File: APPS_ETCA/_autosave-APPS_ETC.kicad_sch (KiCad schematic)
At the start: 7 parts, among them U1 NUCLEO-L432KC, U2 ISO1050DUB, U3 A1365xKTTN-1, U4 A1365xKTTN-1, U5 L78S05CV

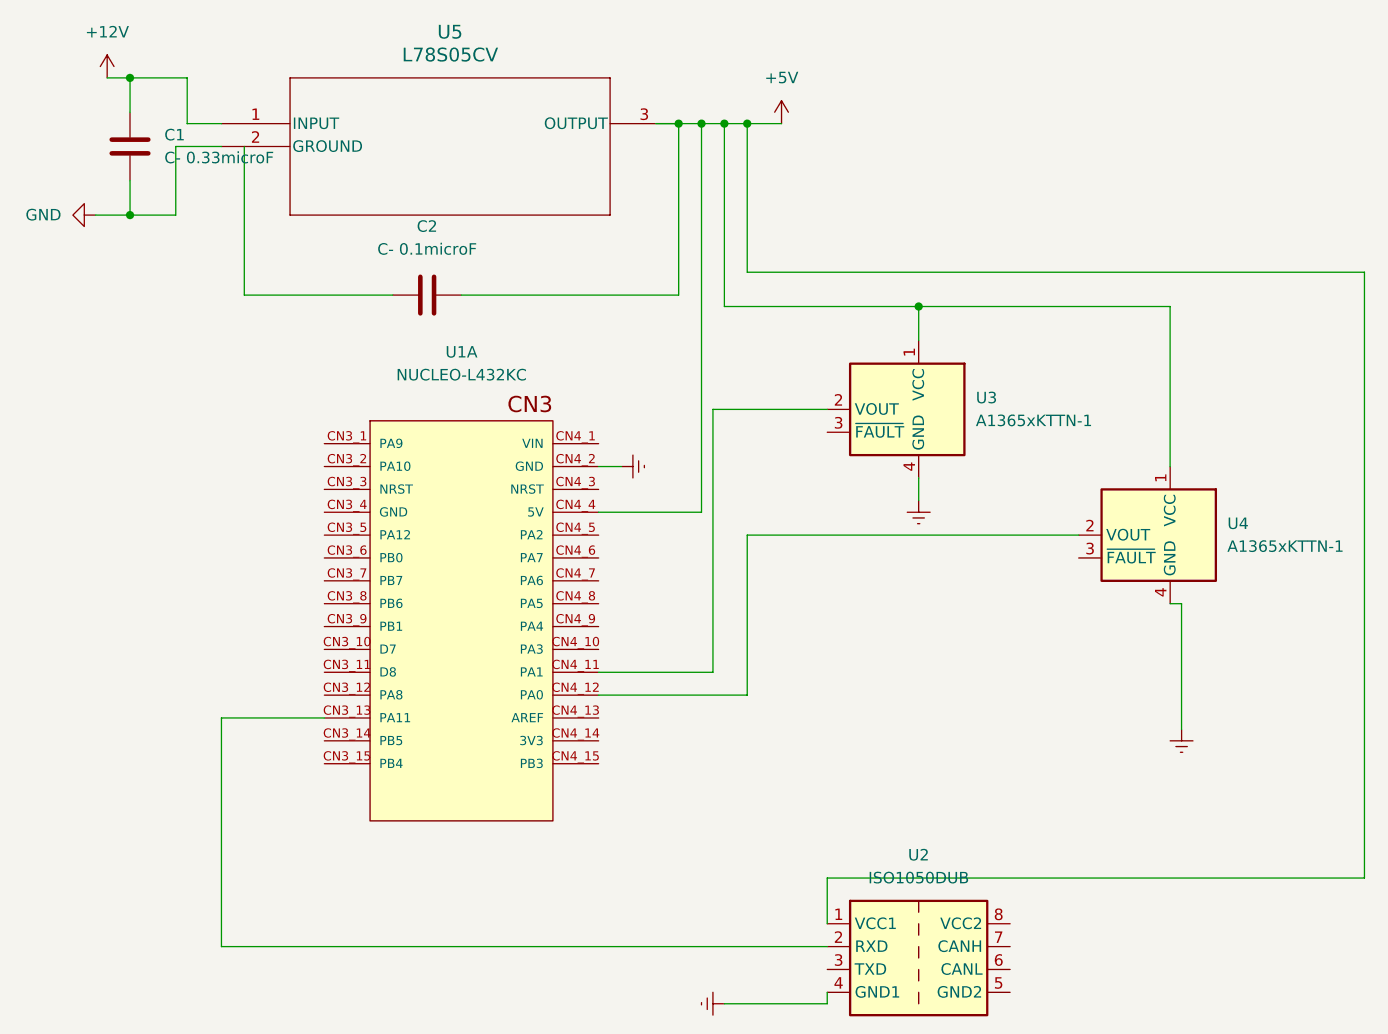
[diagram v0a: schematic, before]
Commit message: schema updates - making progress!
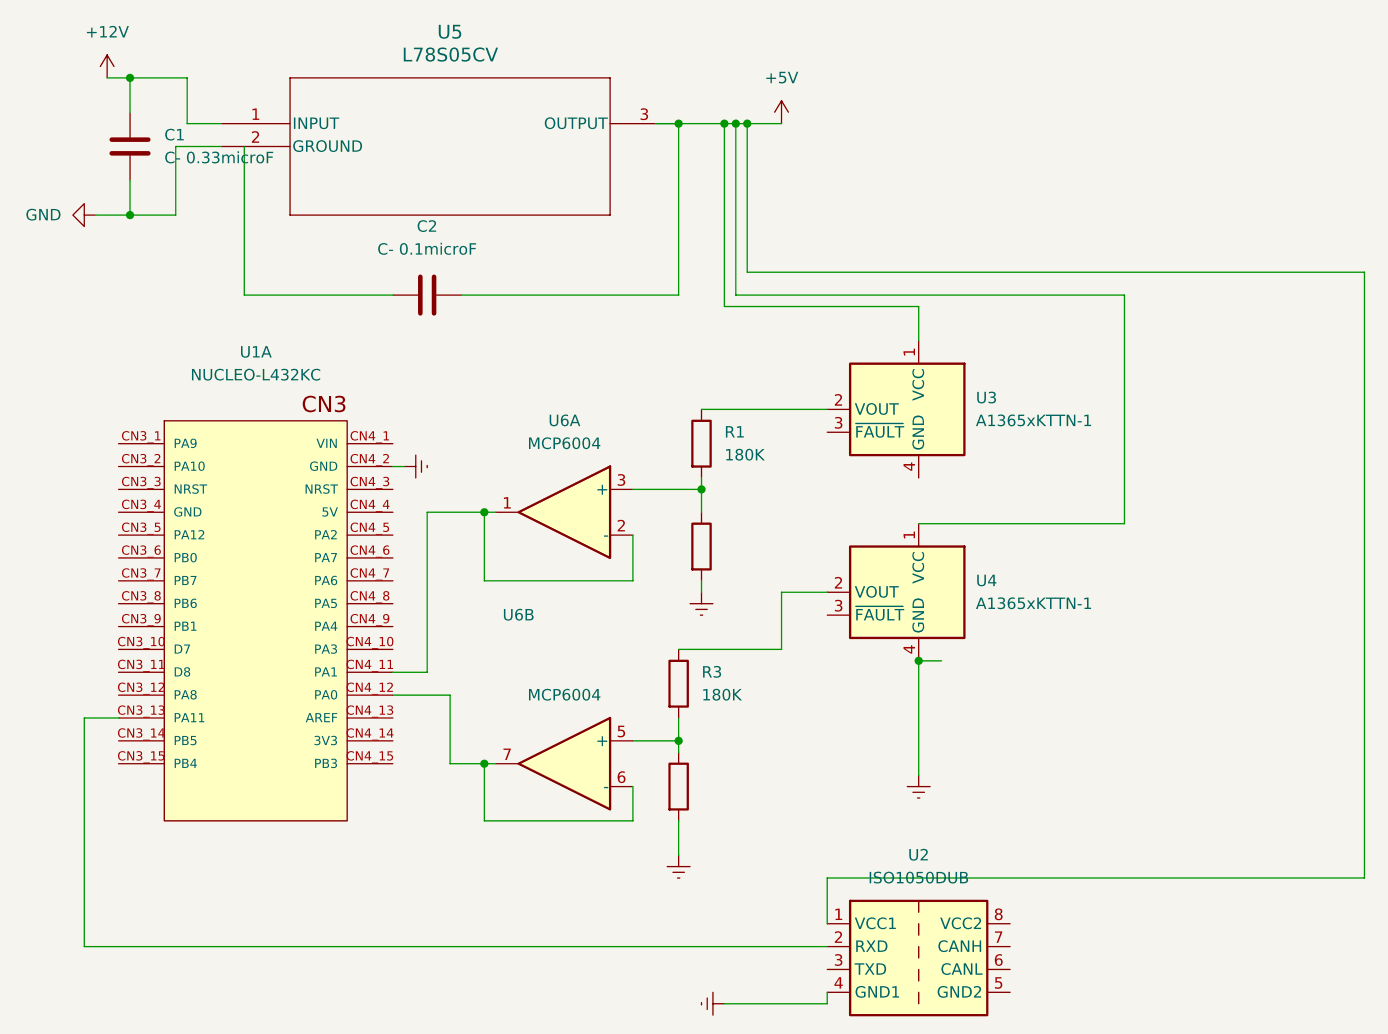
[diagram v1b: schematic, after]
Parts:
- added R1, R3: 180K, symbol Device:R
- added R2, R4: 330k, symbol Device:R
- added U6: MCP6004, symbol Amplifier_Operational:MCP6004
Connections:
- net +5V: no longer U1.CN4_4 (5V)
- net Earth: now also R2.2, R4.2; no longer U3.4 (GND)
- net at U3.2 (VOUT): now also R1.1; no longer U1.CN4_11 (PA1)
- net at U4.2 (VOUT): now also R3.1; no longer U1.CN4_12 (PA0)
- new net: R3.2, R4.1, U6.5 (+)
- new net: U1.CN4_12 (PA0), U6.6 (-), U6.7
- new net: R1.2, R2.1, U6.3 (+)
- new net: U1.CN4_11 (PA1), U6.1, U6.2 (-)
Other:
- moved on the sheet: U1A, U4
